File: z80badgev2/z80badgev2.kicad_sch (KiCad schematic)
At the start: 29 parts, among them J2 Conn_01x20_Pin, J3 Conn_01x20_Pin, SW1 Reset, SW10 Input, SW11 Input, SW2 Input, SW3 Input, SW4 Bus Release, SW5 Power, SW6 Input, SW7 Input, SW8 Input, SW9 Input, U1 Z84C0010P, U2 Z84C20, U3 28C256 SOP28, U4 HM 62256 SOP28, U5 74AHCT1G32, U6 74AHCT1G04, U7 74AHCT1G32, Y1 ACO-xxxMHz

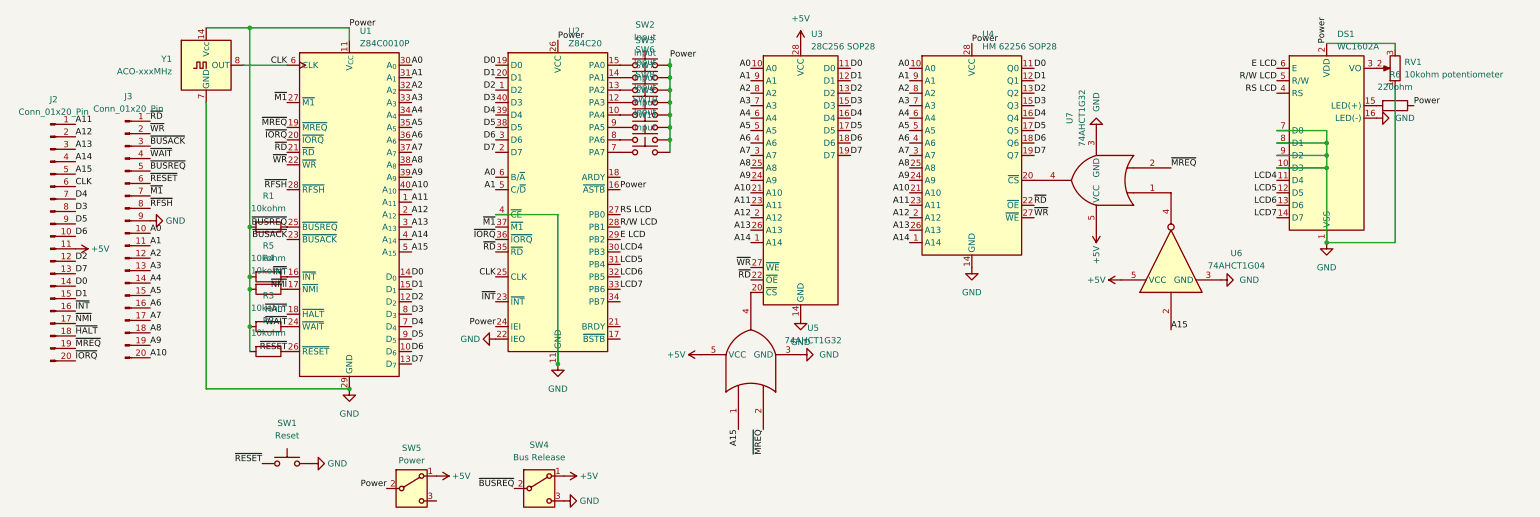
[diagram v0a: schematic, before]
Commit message: Add files via upload
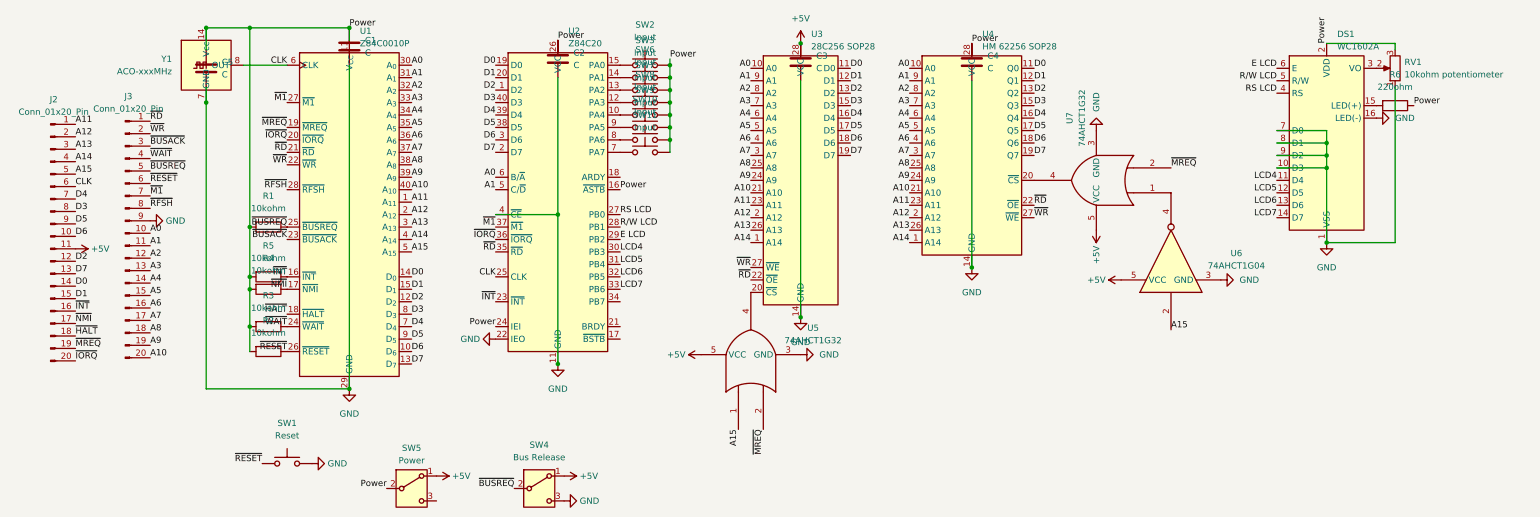
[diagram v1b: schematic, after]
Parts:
- added C1, C2, C3, C4, C5: C, Capacitor_SMD:C_0805_2012Metric, symbol Device:C
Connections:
- net +5V: now also C3.2
- net GND: now also C1.1, C2.1, C3.1, C4.1, C5.1
- net Power: now also C1.2, C2.2, C4.2, C5.2
